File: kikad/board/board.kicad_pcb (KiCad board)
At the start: 2 copper layers, 74.3 x 60 mm, 18 parts, among them J1 Conn_01x10_Socket, J2 Conn_01x10_Socket, J3 Conn_01x06_Socket, J4 Conn_01x02_Socket, J5 Conn_01x02_Socket, Q1 2N3906, Q2 PN2222A, Q3 BC547, Q4 2N3906, U1 TL431LP

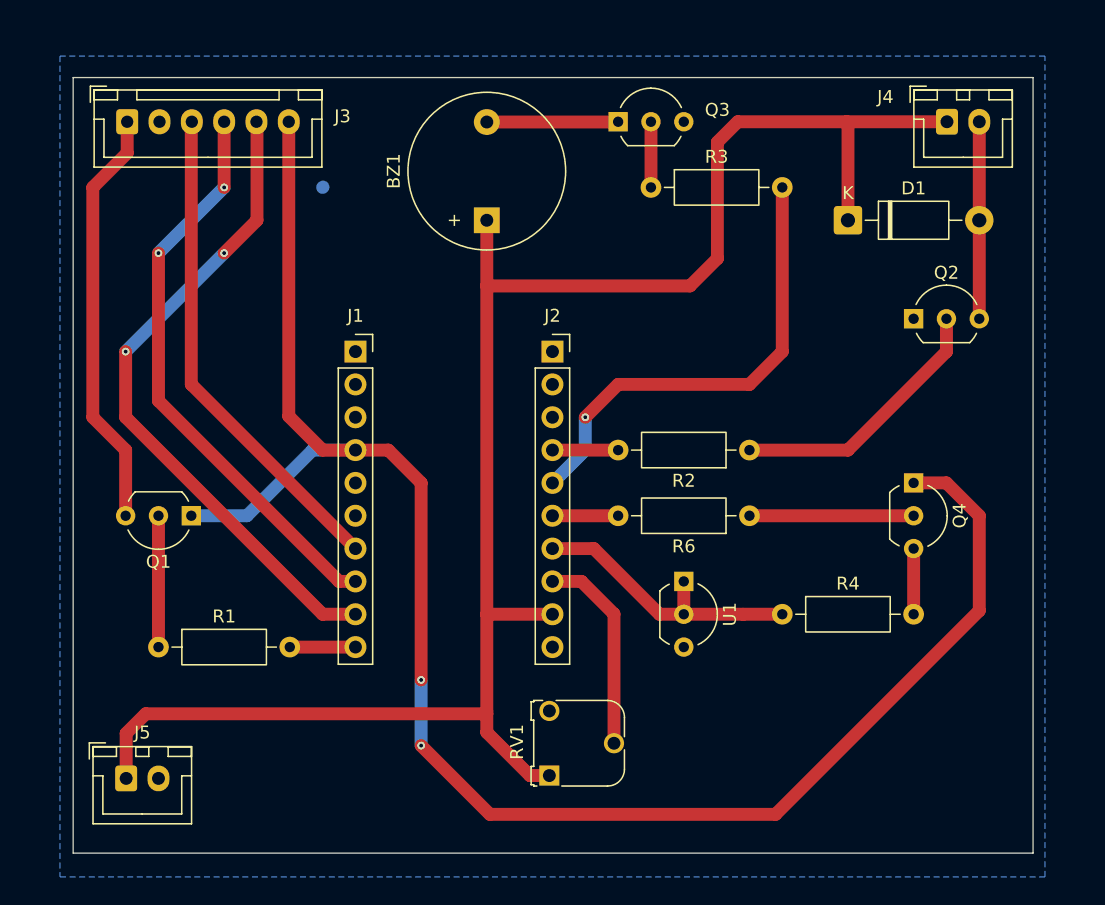
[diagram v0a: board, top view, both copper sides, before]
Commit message: fix design
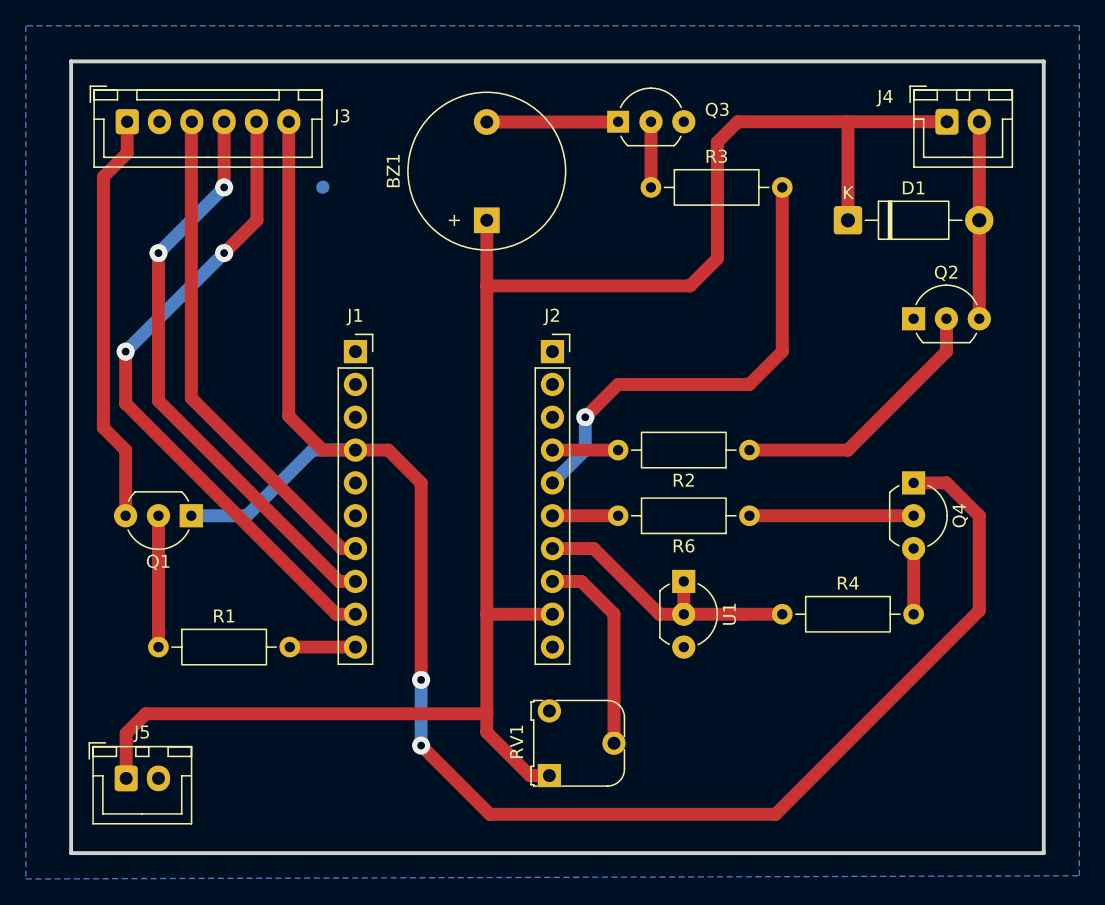
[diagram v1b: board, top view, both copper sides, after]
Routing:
- net /FINGER 3V3: track 32.8 -> 32.1 mm
- net /FINGER_WAKE: track 51.2 -> 50.6 mm
- net /FINGER_RX: track 38.3 -> 38.9 mm
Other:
- board size 74.3 x 60 mm -> 75.2 x 61.2 mm
